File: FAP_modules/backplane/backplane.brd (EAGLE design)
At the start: 160 x 100 mm, 44 parts, among them IC1 REG1117, J1 USB-MICROB, U1 STM32F10XRXT6

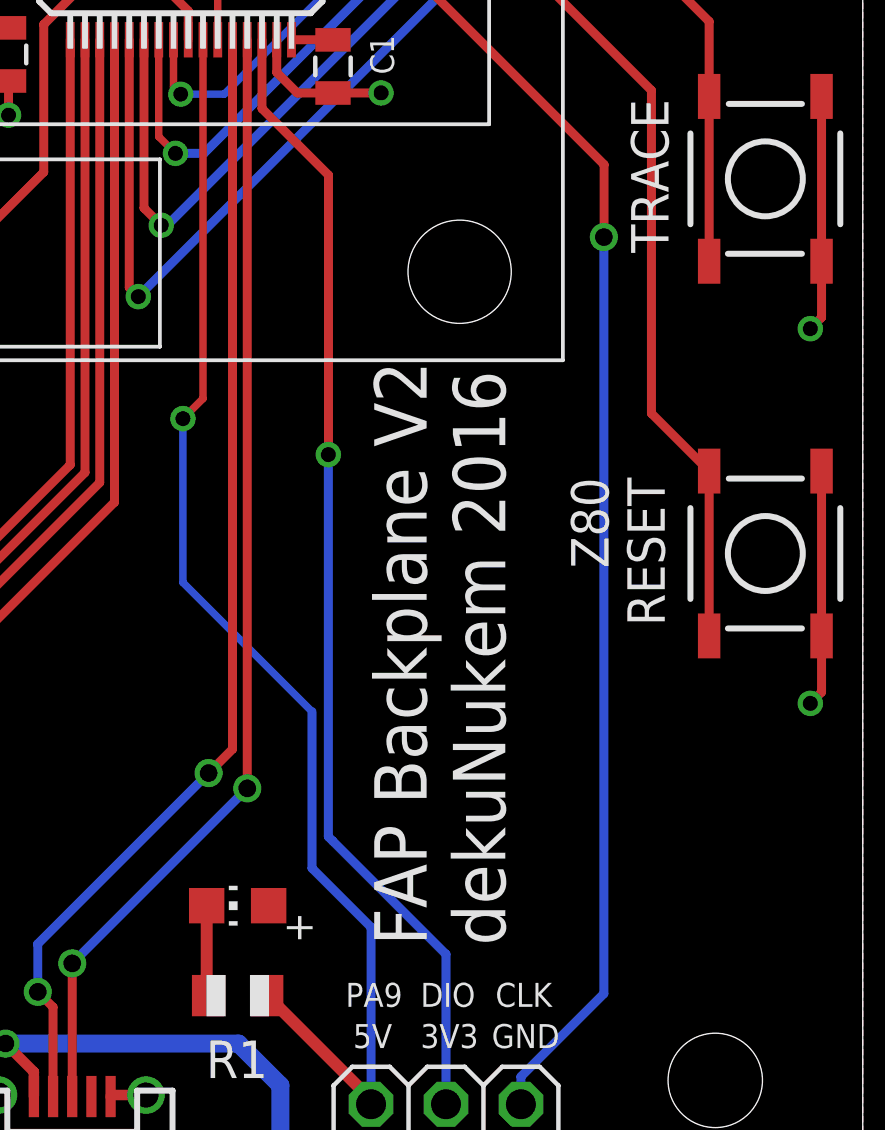
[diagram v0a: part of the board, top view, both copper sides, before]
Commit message: board cleanup
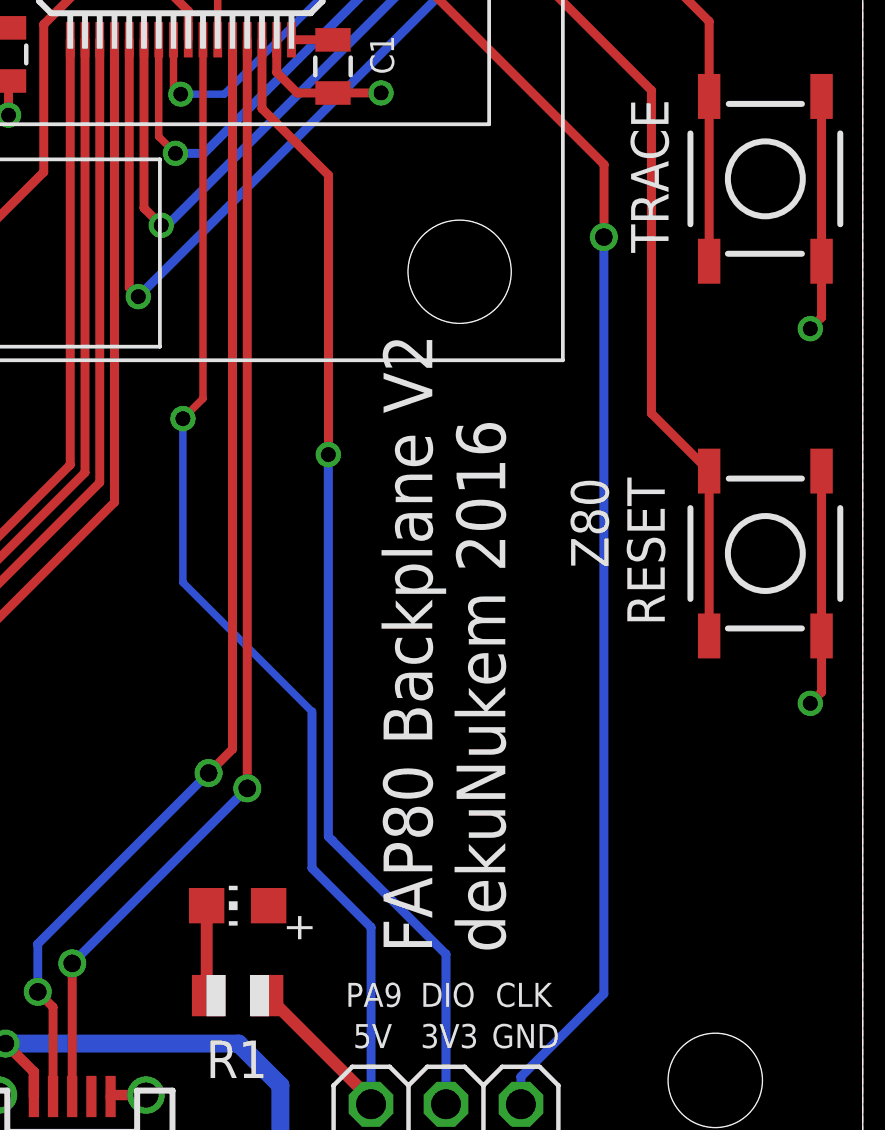
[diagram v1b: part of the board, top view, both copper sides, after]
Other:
- board text added: "FAP80 Backplane V2 dekuNukem 2016"
- board text removed: "FAP Backplane V2 dekuNukem 2016"
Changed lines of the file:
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@@
 <setting verticaltext="up"/>
 </settings>
-<grid distance="1" unitdist="mil" unit="mil" style="lines" multiple="1" display="no" altdistance="0.000123031496" altunitdist="mil" altunit="mil"/>
+<grid distance="10" unitdist="mil" unit="mil" style="lines" multiple="1" display="no" altdistance="0.000123031496" altunitdist="mil" altunit="mil"/>
 <layers>
 <layer number="1" name="Top" color="4" fill="1" visible="yes" active="yes"/>
@@
 <text x="106.152" y="93.6244" size="0.8128" layer="25" rot="R90">RD</text>
 <text x="106.406" y="75.5904" size="0.8128" layer="25" rot="R90">NMI</text>
-<text x="147.8842" y="9.5758" size="1.778" layer="25" rot="R90">FAP Backplane V2
+<text x="147.8842" y="9.3218" size="1.651" layer="25" rot="R90">FAP80 Backplane V2
 dekuNukem 2016</text>
 <text x="14.8082" y="5.8982" size="1.27" layer="25" rot="R180">A15</text>
